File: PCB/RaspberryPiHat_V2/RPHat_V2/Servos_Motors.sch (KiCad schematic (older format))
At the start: 15 parts, among them J10 Conn_01x03, J11 Conn_01x03, J12 Conn_01x03, J13 Conn_01x03, J14 Conn_01x03, J16 Conn_01x06, J5 Conn_01x03, J6 Conn_01x03, J7 Conn_01x03, J8 Conn_01x03, J9 Conn_01x03, SW1 SW_DPDT_x2, U6 Teensy4.0

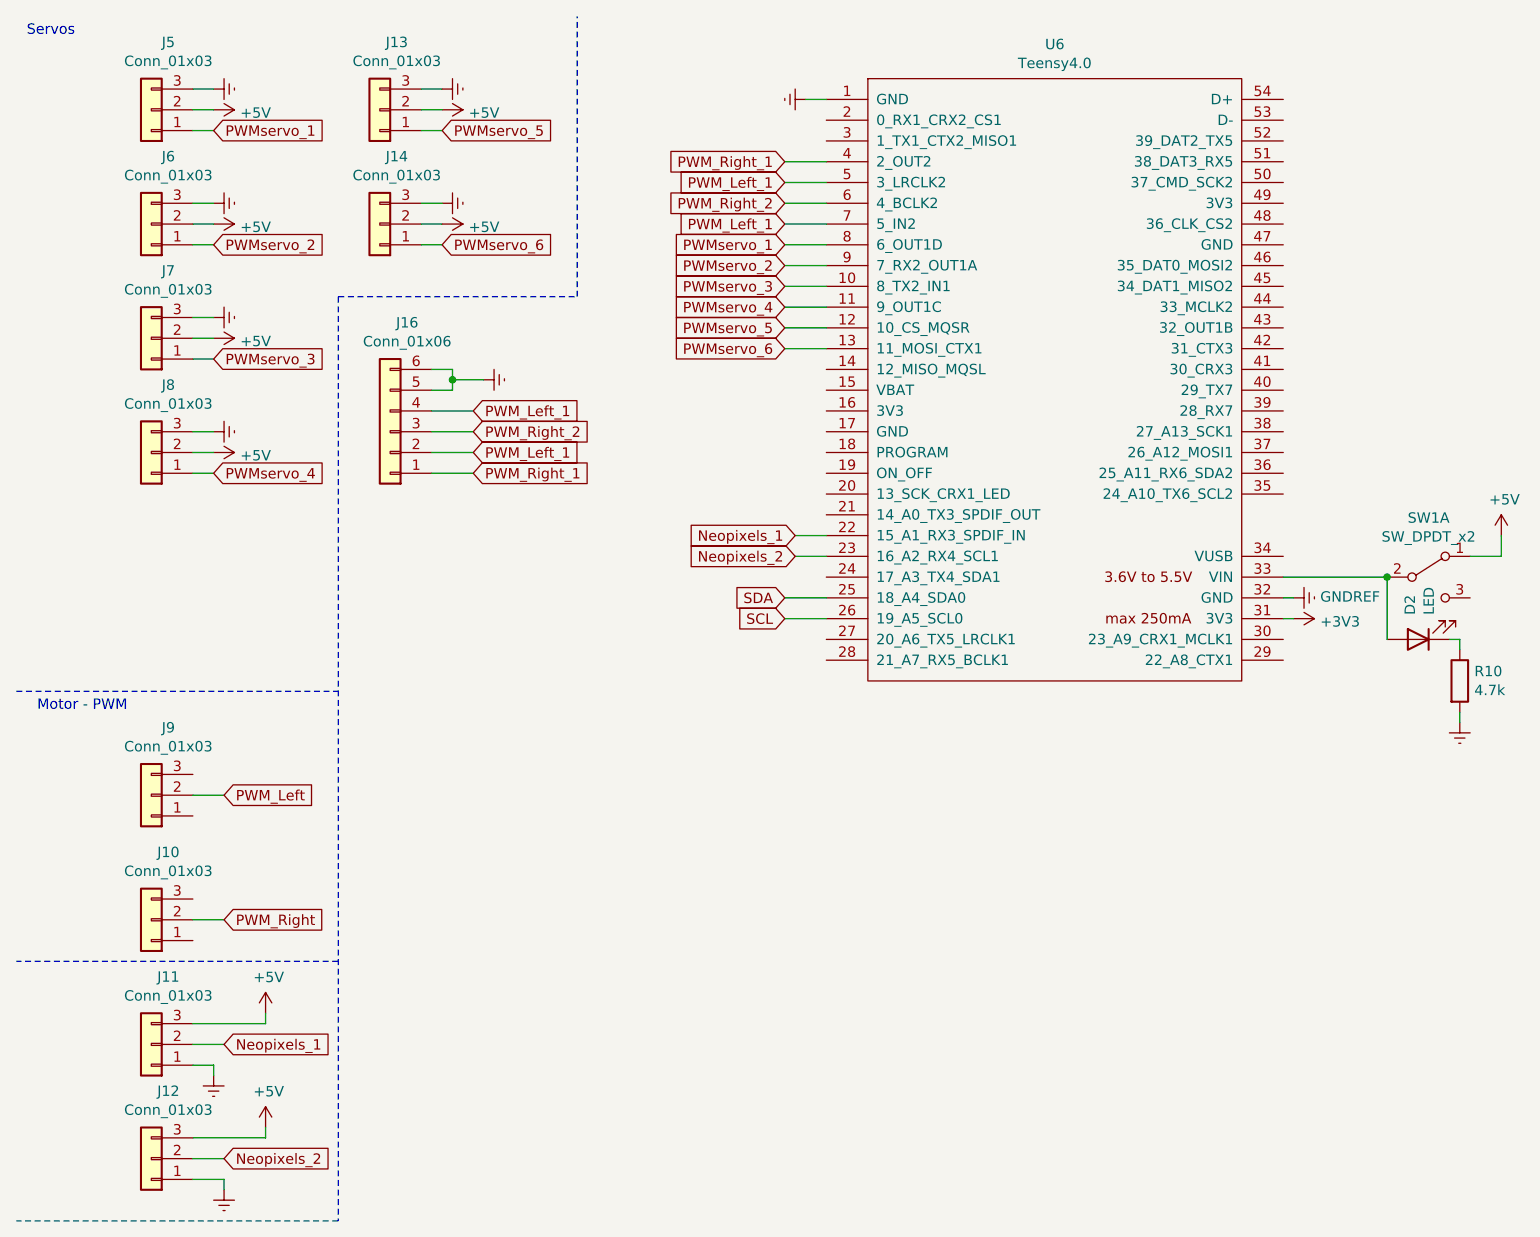
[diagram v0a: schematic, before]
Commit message: working on pcb Ja!
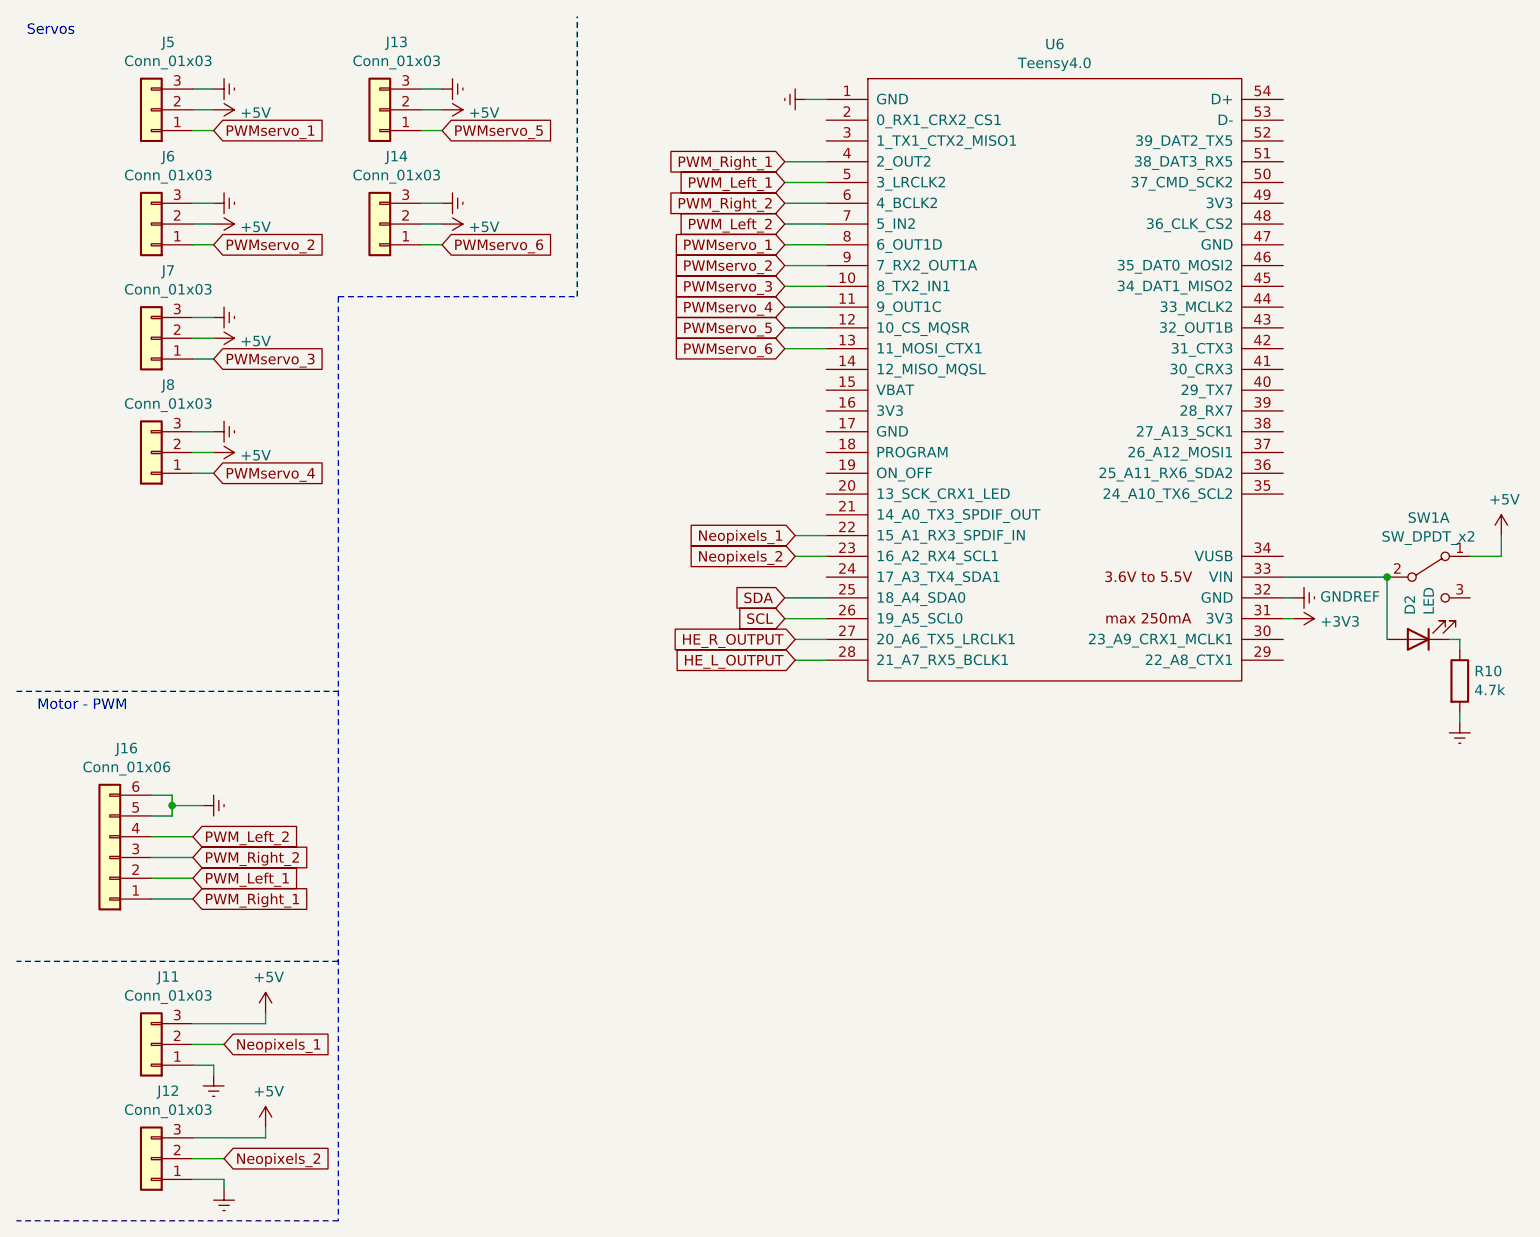
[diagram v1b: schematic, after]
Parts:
- removed J10, J9: Conn_01x03, Connector_PinHeader_2.54mm:PinHeader_1x03_P2.54mm_Vertical, symbol Connector_Generic:Conn_01x03
- J11, J12, J13, J14, J5, J6, J7, J8: footprint Connector_PinHeader_2.54mm:PinHeader_1x03_P2.54mm_Vertical -> Connector_JST:JST_EH_B3B-EH-A_1x03_P2.50mm_Vertical
- J16: footprint Connector_PinHeader_2.54mm:PinHeader_1x06_P2.54mm_Vertical -> Connector_JST:JST_EH_B6B-EH-A_1x06_P2.50mm_Vertical
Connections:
- net PWM_Left_1: no longer J16.4 (Pin_4), U6.7 (5_IN2)
- net HE_R_OUTPUT: now reaches U6.27 (20_A6_TX5_LRCLK1)
- net HE_L_OUTPUT: now reaches U6.28 (21_A7_RX5_BCLK1)
- new net PWM_Left_2: J16.4 (Pin_4), U6.7 (5_IN2)
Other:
- moved on the sheet: J16
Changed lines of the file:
@@
 F 0 "J5" H 1068 625 50  0000 C CNN
 F 1 "Conn_01x03" H 1068 716 50  0000 C CNN
-F 2 "Connector_PinHeader_2.54mm:PinHeader_1x03_P2.54mm_Vertical" H 1150 950 50  0001 C CNN
+F 2 "Connector_JST:JST_EH_B3B-EH-A_1x03_P2.50mm_Vertical" H 1150 950 50  0001 C CNN
 F 3 "~" H 1150 950 50  0001 C CNN
 	1    1150 950
@@
 F 0 "J6" H 1068 1175 50  0000 C CNN
 F 1 "Conn_01x03" H 1068 1266 50  0000 C CNN
-F 2 "Connector_PinHeader_2.54mm:PinHeader_1x03_P2.54mm_Vertical" H 1150 1500 50  0001 C CNN
+F 2 "Connector_JST:JST_EH_B3B-EH-A_1x03_P2.50mm_Vertical" H 1150 1500 50  0001 C CNN
 F 3 "~" H 1150 1500 50  0001 C CNN
 	1    1150 1500
@@
 F 0 "J7" H 1068 1725 50  0000 C CNN
 F 1 "Conn_01x03" H 1068 1816 50  0000 C CNN
-F 2 "Connector_PinHeader_2.54mm:PinHeader_1x03_P2.54mm_Vertical" H 1150 2050 50  0001 C CNN
+F 2 "Connector_JST:JST_EH_B3B-EH-A_1x03_P2.50mm_Vertical" H 1150 2050 50  0001 C CNN
 F 3 "~" H 1150 2050 50  0001 C CNN
 	1    1150 2050
@@
 F 0 "J8" H 1068 2275 50  0000 C CNN
 F 1 "Conn_01x03" H 1068 2366 50  0000 C CNN
-F 2 "Connector_PinHeader_2.54mm:PinHeader_1x03_P2.54mm_Vertical" H 1150 2600 50  0001 C CNN
+F 2 "Connector_JST:JST_EH_B3B-EH-A_1x03_P2.50mm_Vertical" H 1150 2600 50  0001 C CNN
 F 3 "~" H 1150 2600 50  0001 C CNN
 	1    1150 2600
@@
 F 0 "J13" H 2168 625 50  0000 C CNN
 F 1 "Conn_01x03" H 2168 716 50  0000 C CNN
-F 2 "Connector_PinHeader_2.54mm:PinHeader_1x03_P2.54mm_Vertical" H 2250 950 50  0001 C CNN
+F 2 "Connector_JST:JST_EH_B3B-EH-A_1x03_P2.50mm_Vertical" H 2250 950 50  0001 C CNN
 F 3 "~" H 2250 950 50  0001 C CNN
 	1    2250 950
@@
 F 0 "J14" H 2168 1175 50  0000 C CNN
 F 1 "Conn_01x03" H 2168 1266 50  0000 C CNN
-F 2 "Connector_PinHeader_2.54mm:PinHeader_1x03_P2.54mm_Vertical" H 2250 1500 50  0001 C CNN
+F 2 "Connector_JST:JST_EH_B3B-EH-A_1x03_P2.50mm_Vertical" H 2250 1500 50  0001 C CNN
 F 3 "~" H 2250 1500 50  0001 C CNN
 	1    2250 1500
@@
 Text Notes 550  600  0    50   ~ 0
 Servos\n
-$Comp
-L Connector_Generic:Conn_01x03 J9
-U 1 1 609A3D4E
-P 1150 4250
-F 0 "J9" H 1068 3925 50  0000 C CNN
-F 1 "Conn_01x03" H 1068 4016 50  0000 C CNN
-F 2 "Connector_PinHeader_2.54mm:PinHeader_1x03_P2.54mm_Vertical" H 1150 4250 50  0001 C CNN
-F 3 "~" H 1150 4250 50  0001 C CNN
-	1    1150 4250
-	-1   0    0    1
-$EndComp
-$Comp
-L Connector_Generic:Conn_01x03 J10
-U 1 1 609A3F8F
-P 1150 4850
-F 0 "J10" H 1068 4525 50  0000 C CNN
-F 1 "Conn_01x03" H 1068 4616 50  0000 C CNN
-F 2 "Connector_PinHeader_2.54mm:PinHeader_1x03_P2.54mm_Vertical" H 1150 4850 50  0001 C CNN
-F 3 "~" H 1150 4850 50  0001 C CNN
-	1    1150 4850
-	-1   0    0    1
-$EndComp
-Text Notes 600  3850 0    50   ~ 0
-Motor - PWM
 $Comp
 L power:GNDREF #PWR0143
@@
 Wire Wire Line
 	2450 1600 2550 1600
-Text GLabel 1500 4250 2    50   Input ~ 0
-PWM_Left
-Text GLabel 1500 4850 2    50   Input ~ 0
-PWM_Right
-Wire Wire Line
-	1500 4250 1350 4250
-Wire Wire Line
-	1500 4850 1350 4850
 Wire Notes Line
 	2050 5050 500  5050
@@
 F 0 "J11" H 1068 5125 50  0000 C CNN
 F 1 "Conn_01x03" H 1068 5216 50  0000 C CNN
-F 2 "Connector_PinHeader_2.54mm:PinHeader_1x03_P2.54mm_Vertical" H 1150 5450 50  0001 C CNN
+F 2 "Connector_JST:JST_EH_B3B-EH-A_1x03_P2.50mm_Vertical" H 1150 5450 50  0001 C CNN
 F 3 "~" H 1150 5450 50  0001 C CNN
 	1    1150 5450
@@
 F 0 "J12" H 1068 5675 50  0000 C CNN
 F 1 "Conn_01x03" H 1068 5766 50  0000 C CNN
-F 2 "Connector_PinHeader_2.54mm:PinHeader_1x03_P2.54mm_Vertical" H 1150 6000 50  0001 C CNN
+F 2 "Connector_JST:JST_EH_B3B-EH-A_1x03_P2.50mm_Vertical" H 1150 6000 50  0001 C CNN
 F 3 "~" H 1150 6000 50  0001 C CNN
 	1    1150 6000
@@
 PWM_Right_2
 Text GLabel 4200 1500 0    50   Input ~ 0
-PWM_Left_1
+PWM_Left_2
 Wire Wire Line
 	4200 1500 4400 1500
@@
 L Connector_Generic:Conn_01x06 J16
 U 1 1 60B35E0D
-P 2300 2500
-F 0 "J16" H 2218 1975 50  0000 C CNN
-F 1 "Conn_01x06" H 2218 2066 50  0000 C CNN
-F 2 "Connector_PinHeader_2.54mm:PinHeader_1x06_P2.54mm_Vertical" H 2300 2500 50  0001 C CNN
-F 3 "~" H 2300 2500 50  0001 C CNN
-	1    2300 2500
-	-1   0    0    1
-$EndComp
-Text GLabel 2700 2700 2    50   Input ~ 0
+P 950 4550
+F 0 "J16" H 868 4025 50  0000 C CNN
+F 1 "Conn_01x06" H 868 4116 50  0000 C CNN
+F 2 "Connector_JST:JST_EH_B6B-EH-A_1x06_P2.50mm_Vertical" H 950 4550 50  0001 C CNN
+F 3 "~" H 950 4550 50  0001 C CNN
+	1    950  4550
+	-1   0    0    1
+$EndComp
+Text GLabel 1350 4750 2    50   Input ~ 0
 PWM_Right_1
-Text GLabel 2700 2600 2    50   Input ~ 0
+Text GLabel 1350 4650 2    50   Input ~ 0
 PWM_Left_1
 Wire Wire Line
-	2700 2600 2500 2600
-Wire Wire Line
-	2700 2700 2500 2700
-Text GLabel 2700 2500 2    50   Input ~ 0
+	1350 4650 1150 4650
+Wire Wire Line
+	1350 4750 1150 4750
+Text GLabel 1350 4550 2    50   Input ~ 0
 PWM_Right_2
-Text GLabel 2700 2400 2    50   Input ~ 0
-PWM_Left_1
-Wire Wire Line
-	2700 2400 2500 2400
-Wire Wire Line
-	2700 2500 2500 2500
+Text GLabel 1350 4450 2    50   Input ~ 0
+PWM_Left_2
+Wire Wire Line
+	1350 4450 1150 4450
+Wire Wire Line
+	1350 4550 1150 4550
 $Comp
 L power:GNDREF #PWR03
 U 1 1 60B40966
-P 2750 2250
-F 0 "#PWR03" H 2750 2000 50  0001 C CNN
-F 1 "GNDREF" V 2755 2122 50  0001 R CNN
-F 2 "" H 2750 2250 50  0001 C CNN
-F 3 "" H 2750 2250 50  0001 C CNN
-	1    2750 2250
-	0    -1   -1   0
-$EndComp
-Wire Wire Line
-	2500 2200 2600 2200
-Wire Wire Line
-	2600 2200 2600 2250
-Wire Wire Line
-	2600 2250 2750 2250
-Wire Wire Line
-	2500 2300 2600 2300
-Wire Wire Line
-	2600 2300 2600 2250
-Connection ~ 2600 2250
+P 1400 4300
+F 0 "#PWR03" H 1400 4050 50  0001 C CNN
+F 1 "GNDREF" V 1405 4172 50  0001 R CNN
+F 2 "" H 1400 4300 50  0001 C CNN
+F 3 "" H 1400 4300 50  0001 C CNN
+	1    1400 4300
+	0    -1   -1   0
+$EndComp
+Wire Wire Line
+	1150 4250 1250 4250
+Wire Wire Line
+	1250 4250 1250 4300
+Wire Wire Line
+	1250 4300 1400 4300
+Wire Wire Line
+	1150 4350 1250 4350
+Wire Wire Line
+	1250 4350 1250 4300
+Connection ~ 1250 4300
 Text GLabel 4250 3000 0    50   Input ~ 0
 Neopixels_1
@@
 Wire Wire Line
 	6600 3200 7100 3200
+Text Notes 600  3850 0    50   ~ 0
+Motor - PWM
+Text GLabel 4250 3500 0    50   Input ~ 0
+HE_R_OUTPUT
+Text GLabel 4250 3600 0    50   Input ~ 0
+HE_L_OUTPUT
+Wire Wire Line
+	4250 3600 4400 3600
+Wire Wire Line
+	4250 3500 4400 3500
 $EndSCHEMATC
